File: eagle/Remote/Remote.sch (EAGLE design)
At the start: 13 parts, among them IC1 ATMEGA325P

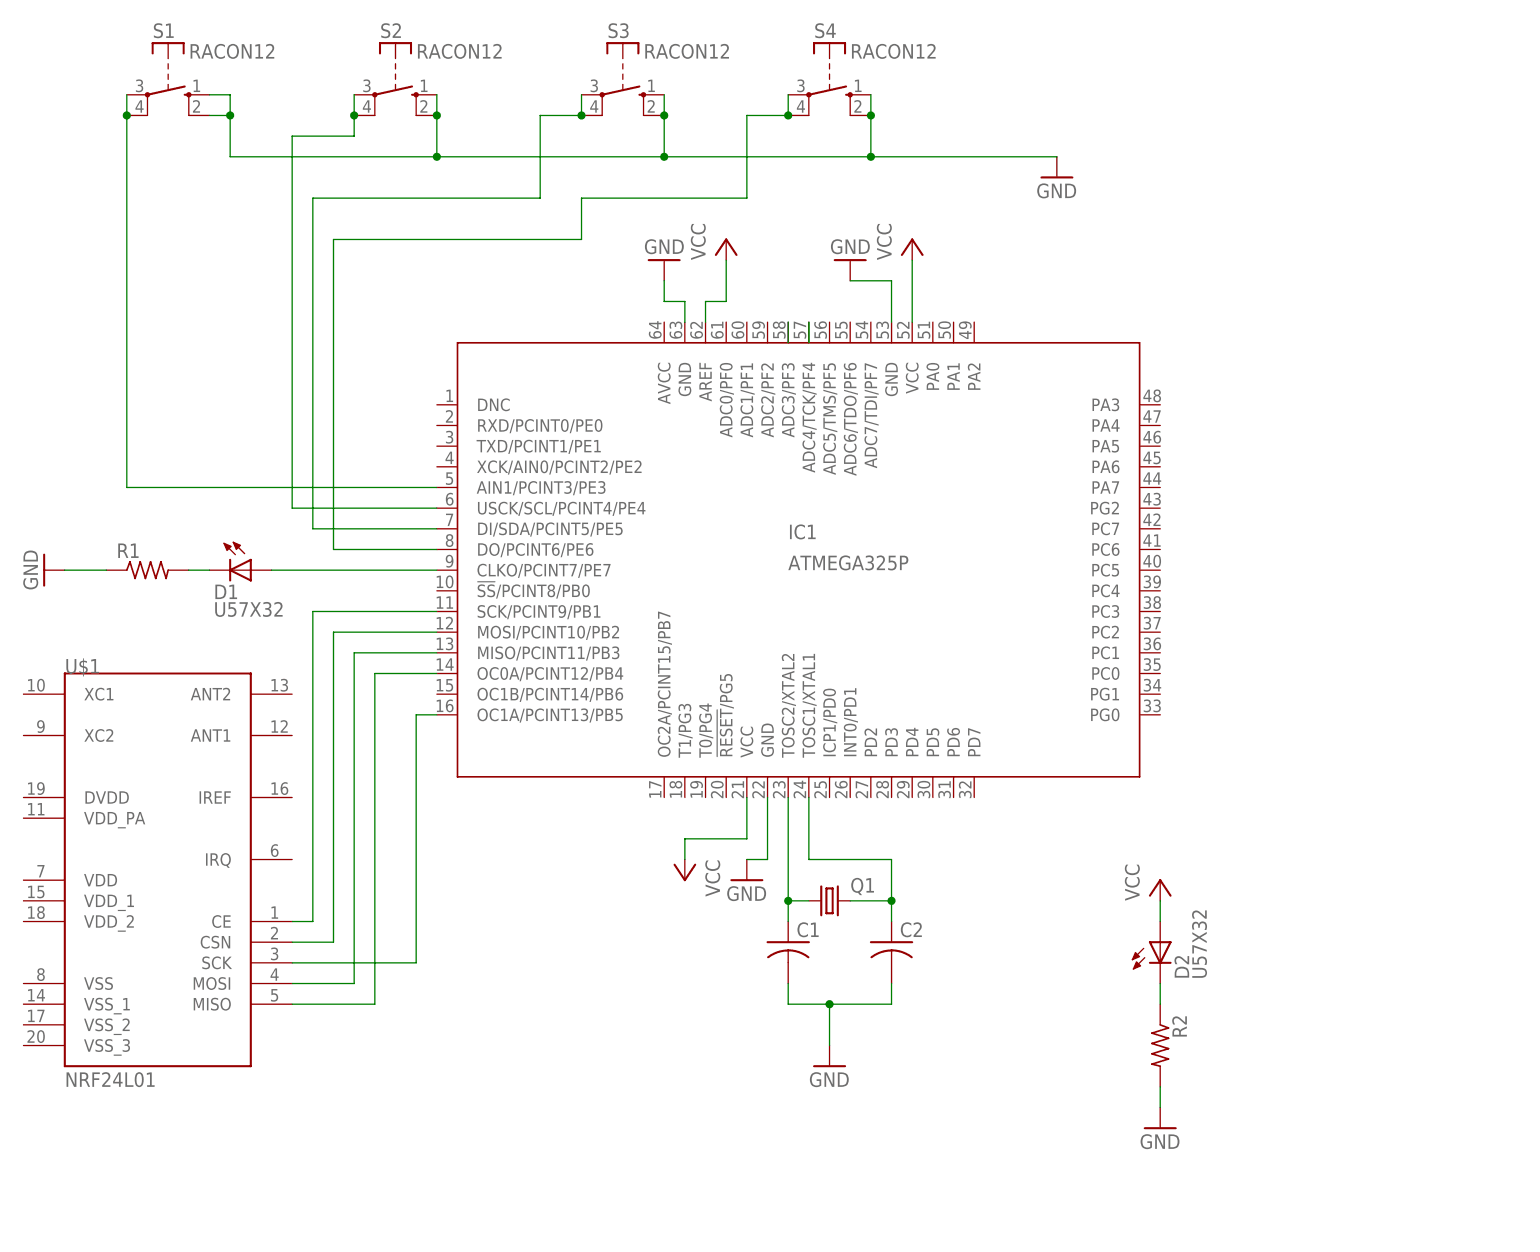
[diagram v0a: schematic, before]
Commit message: update schematic and implement board
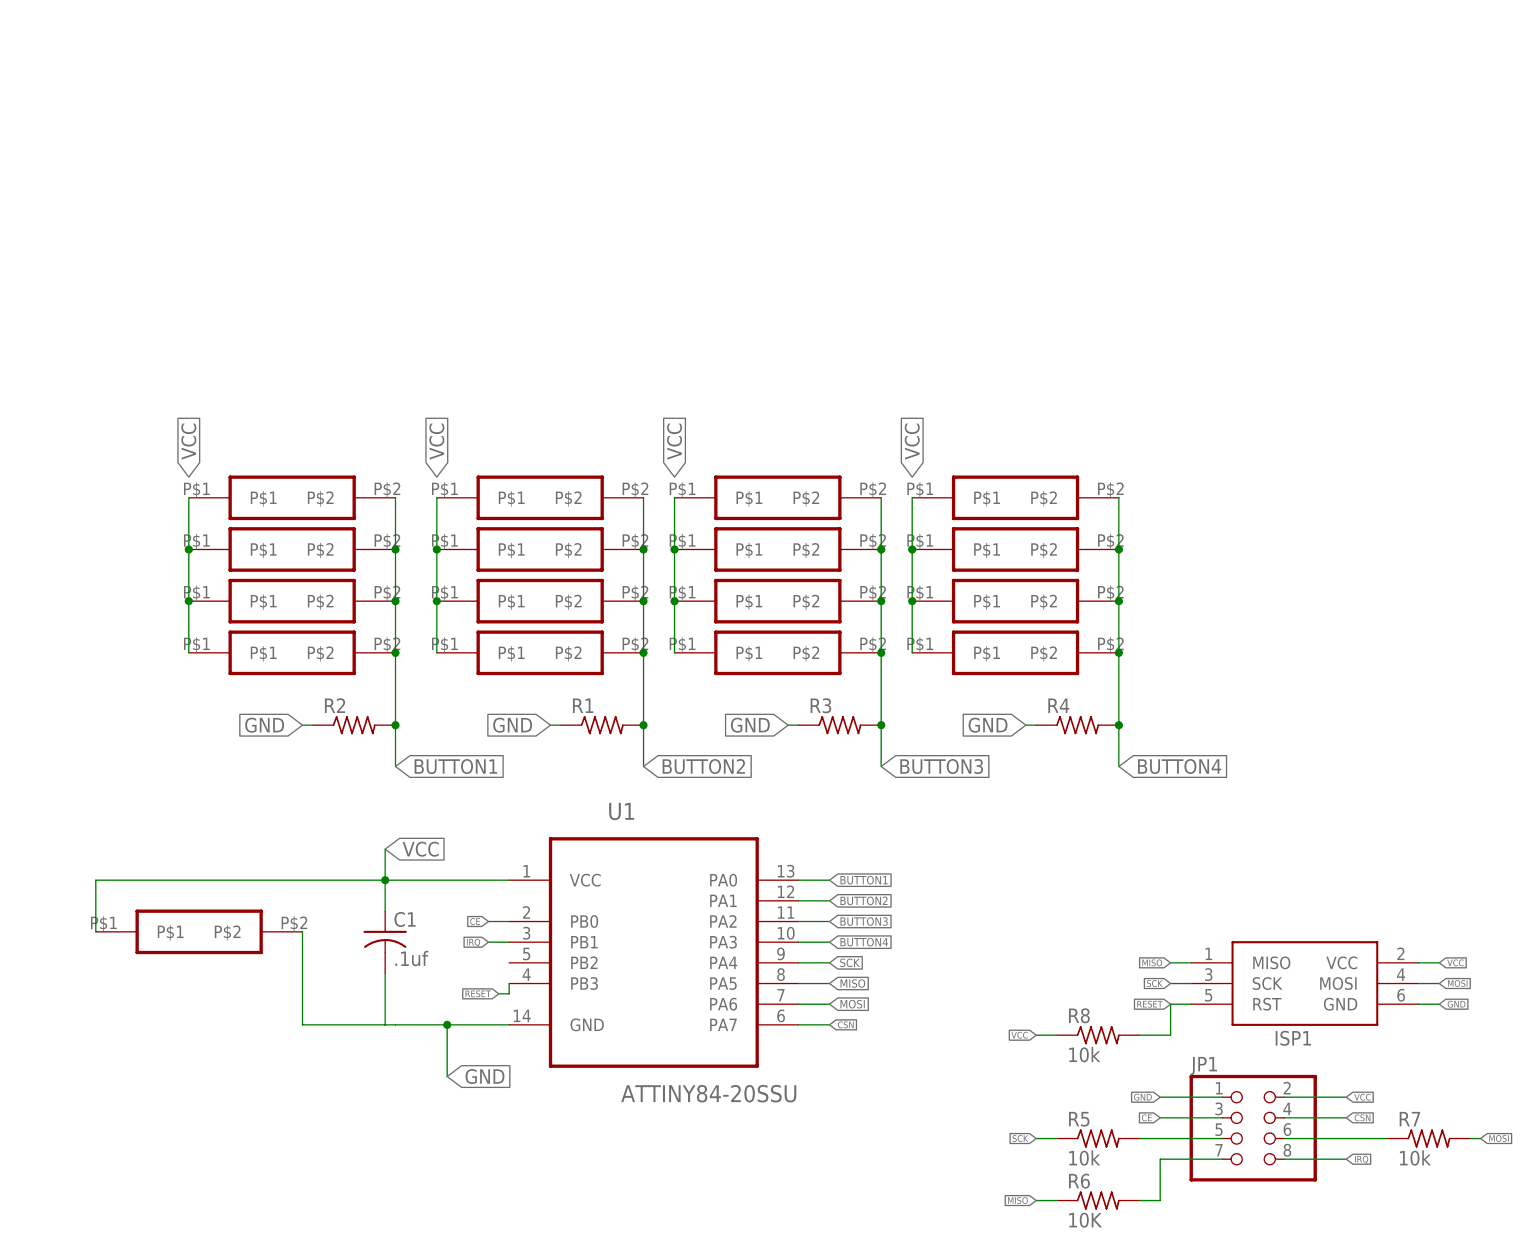
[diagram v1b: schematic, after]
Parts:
- removed C2: (no value), resistor:C-US025-024X044
- removed D1, D2: U57X32, led:U57X32
- removed IC1: ATMEGA325P, atmel:ATMEGA325P
- removed Q1: (no value), crystal:CRYSTALHC49S
- removed S1, S2, S3, S4: RACON12, switch-misc:RACON12
- added BUTTON1-A, BUTTON1-B, BUTTON1-C, BUTTON1-D, BUTTON2-A, BUTTON2-B, BUTTON2-C, BUTTON2-D, BUTTON3-A, BUTTON3-B, BUTTON3-C, BUTTON3-D, BUTTON4-A, BUTTON4-B, BUTTON4-C, BUTTON4-D: BUTTON-25MM-4PAD, solids:BUTTON-25MM-4PAD
- added ISP1: AVRISP-6, adafruit:AVRISP-6
- added JP1: (no value), pinhead:PINHD-2X4
- added R3, R4: (no value), adafruit:R-US_R0805
- added R5, R7, R8: 10k, adafruit:R-US_R0805
- added R6: 10K, adafruit:R-US_R0805
- added U1: ATTINY84-20SSU, Atmel_By_element14_Batch_1:ATTINY84-20SSU
- C1: value (none) -> .1uf; device resistor:C-US025-024X044 -> adafruit:C-USC0805
- R1, R2: device resistor:R-US_0204/5 -> adafruit:R-US_R0805
- U$1: value NRF24L01 -> A99327CT-ND; device nrf24l01:NRF24L01 -> solids:A99327CT-ND
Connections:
- removed net N$1: IC1.SCK/PCINT9/PB1, U$1.CE
- removed net N$10: IC1.ADC3/PF3
- removed net N$11: IC1.OC0A/PCINT12/PB4, U$1.MISO
- removed net N$12: C1.1, IC1.TOSC2/XTAL2, Q1.1
- removed net N$13: IC1.AIN1/PCINT3/PE3, S1.P, S1.P@1
- removed net N$14: IC1.USCK/SCL/PCINT4/PE4, S2.P, S2.P@1
- removed net N$15: IC1.DI/SDA/PCINT5/PE5, S3.P, S3.P@1
- removed net N$16: IC1.DO/PCINT6/PE6, S4.P, S4.P@1
- removed net N$17: C2.1, IC1.TOSC1/XTAL1, Q1.2
- removed net N$5: D1.C, R1.2
- removed net N$7: IC1.OC1A/PCINT13/PB5, U$1.SCK
- removed net N$8: IC1.MISO/PCINT11/PB3, U$1.MOSI
- removed net N$9: D1.A, IC1.CLKO/PCINT7/PE7
- new net BUTTON1: BUTTON1-A.P$2, BUTTON1-B.P$2, BUTTON1-C.P$2, BUTTON1-D.P$2, R2.2, U1.PA0
- new net BUTTON2: BUTTON2-A.P$2, BUTTON2-B.P$2, BUTTON2-C.P$2, BUTTON2-D.P$2, R1.2, U1.PA1
- new net BUTTON3: BUTTON3-A.P$2, BUTTON3-B.P$2, BUTTON3-C.P$2, BUTTON3-D.P$2, R3.2, U1.PA2
- new net BUTTON4: BUTTON4-A.P$2, BUTTON4-B.P$2, BUTTON4-C.P$2, BUTTON4-D.P$2, R4.2, U1.PA3
- new net CE: JP1.3, U1.PB0
- new net CSN: JP1.4, U1.PA7
- new net IRQ: JP1.8, U1.PB1
- new net MISO: ISP1.MISO, R6.1, U1.PA5
- new net MOSI: ISP1.MOSI, R7.2, U1.PA6
- new net RESET: ISP1.RST, R8.2, U1.PB3
- new net SCK: ISP1.SCK, R5.1, U1.PA4
- net GND: now also ISP1.GND, JP1.1, R2.1, R3.1, R4.1, U$1.P$2, U1.GND; no longer C2.2, IC1.GND, IC1.GND@1, IC1.GND@2, R2.2, S1.S, S1.S@1, S2.S, S2.S@1, S3.S, S3.S@1, S4.S, S4.S@1
- net N$2: now also JP1.5, R5.2; no longer IC1.MOSI/PCINT10/PB2, U$1.CSN
- net N$3: now also JP1.7, R6.2; no longer D2.C, R2.1
- net N$4: now also JP1.6, R7.1; no longer IC1.ADC4/TCK/PF4
- net VCC: now also BUTTON1-A.P$1, BUTTON1-B.P$1, BUTTON1-C.P$1, BUTTON1-D.P$1, BUTTON2-A.P$1, BUTTON2-B.P$1, BUTTON2-C.P$1, BUTTON2-D.P$1, BUTTON3-A.P$1, BUTTON3-B.P$1, BUTTON3-C.P$1, BUTTON3-D.P$1, BUTTON4-A.P$1, BUTTON4-B.P$1, BUTTON4-C.P$1, BUTTON4-D.P$1, C1.1, ISP1.VCC, JP1.2, R8.1, U$1.P$1, U1.VCC; no longer D2.A, IC1.AREF, IC1.VCC, IC1.VCC@1
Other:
- moved on the sheet: C1, R1, R2
